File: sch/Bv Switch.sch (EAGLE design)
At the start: 34 parts, among them IC1 FT232RL, IC2 7805, IC3 MEGA8-AI, IC4 74HCT595D, J2 USBHD

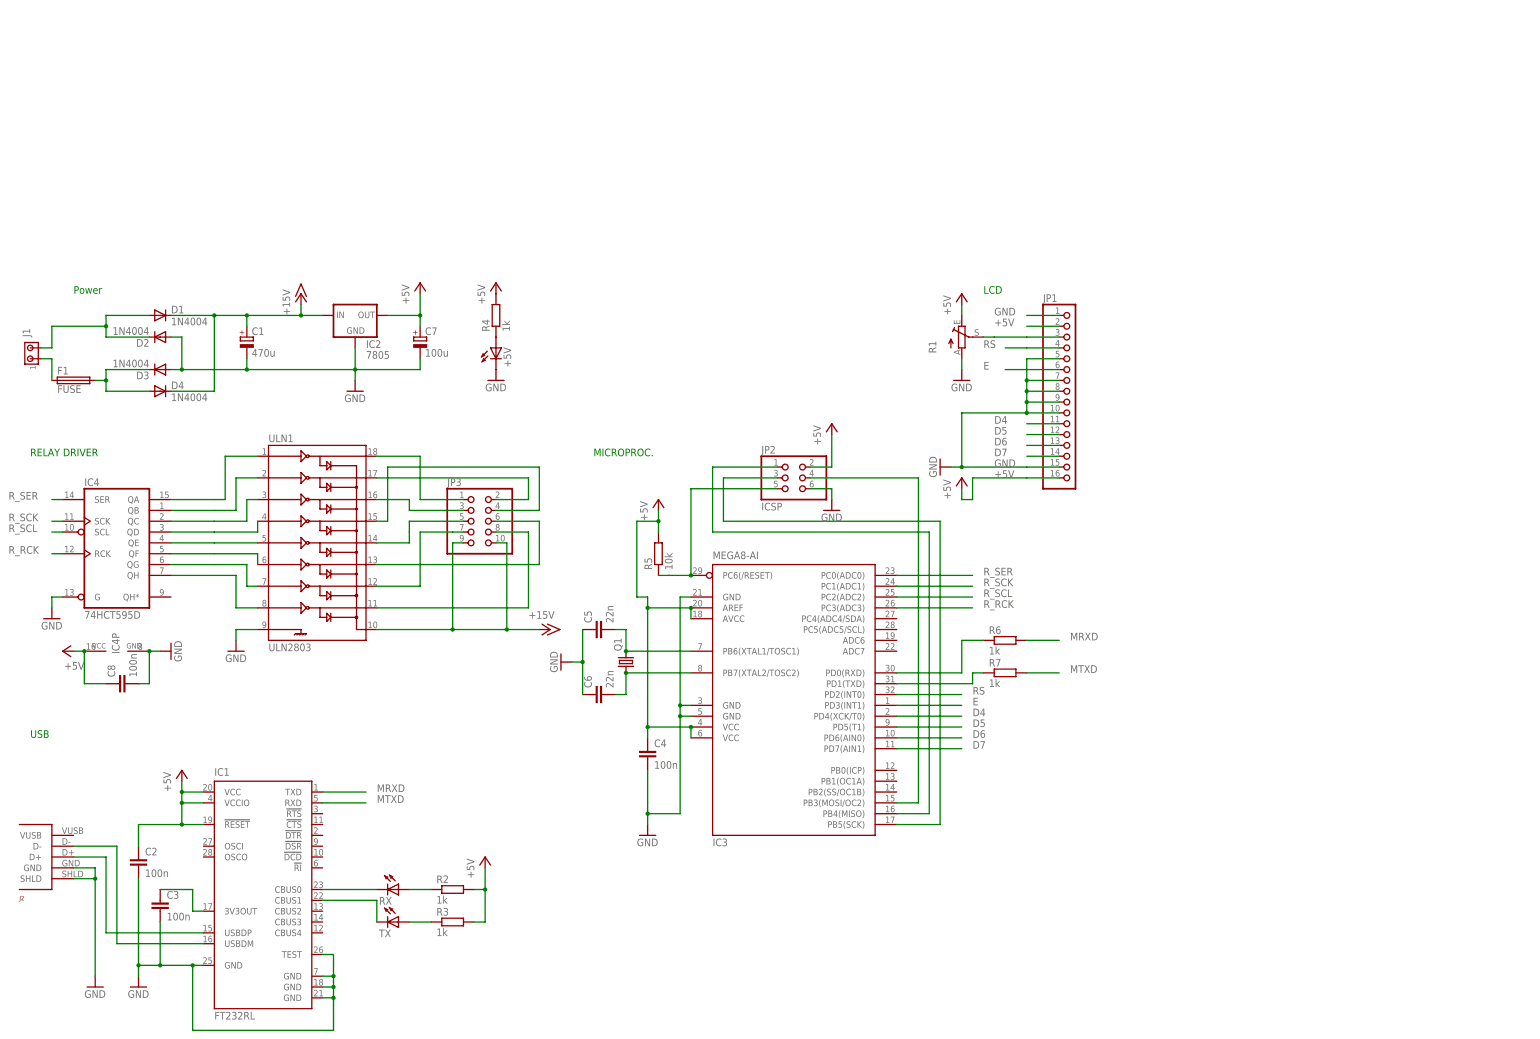
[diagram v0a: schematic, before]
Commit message: Reset implementation, initial BRD
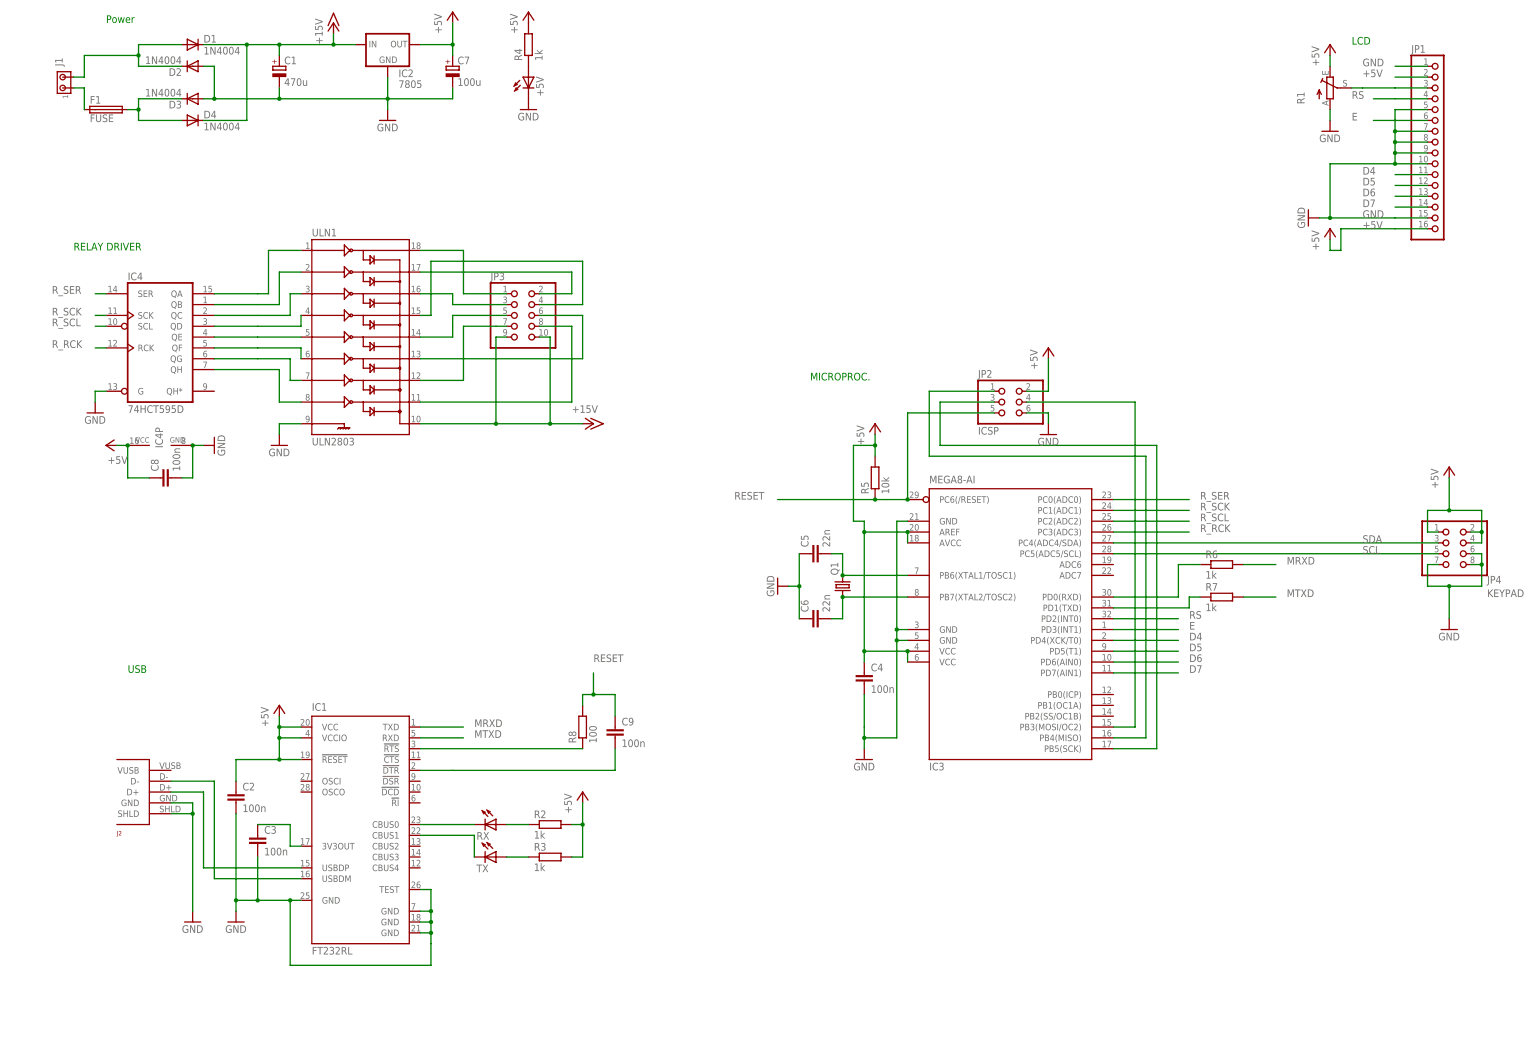
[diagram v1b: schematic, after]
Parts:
- added C9: 100n, rcl:C-EUC1206
- added JP4: KEYPAD, pinhead:PINHD-2X4
- added R8: 100, rcl:R-EU_R1206
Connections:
- removed net N$9: IC3.PC6(/RESET), JP2.5, R5.1
- new net N$36: C9.2, IC1.!DTR
- new net N$37: IC1.!RTS, R8.1
- new net RESET: C9.1, IC3.PC6(/RESET), JP2.5, R5.1, R8.2
- new net SCL: IC3.PC5(ADC5/SCL), JP4.5
- new net SDA: IC3.PC4(ADC4/SDA), JP4.3
- net +5V: now also JP4.1, JP4.2, JP4.4
- net GND: now also JP4.6, JP4.7, JP4.8
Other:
- moved on the sheet: +5V, C1, C2, C3, C4, C5, C6, C7, C8, D1, D2, D3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
